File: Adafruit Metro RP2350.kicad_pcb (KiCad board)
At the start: 4 copper layers, 55 x 65.6 mm, 64 parts, among them J1 USB_C_Receptacle_USB2.0_14P, J2 Conn_02x09_Counter_Clockwise, J3 Conn_01x05_Pin, SW2 SW_RA, SW3 SW_RA, U1 APS1604M-3SQRx-SN, U2 W25Q128JVS, U4 74LVC1G19, U5 NCP1117-3.3_SOT223, U7 APS1604M-3SQRx-SN, X4 RP2350B, Y1 12MHz_10pF_50ohm

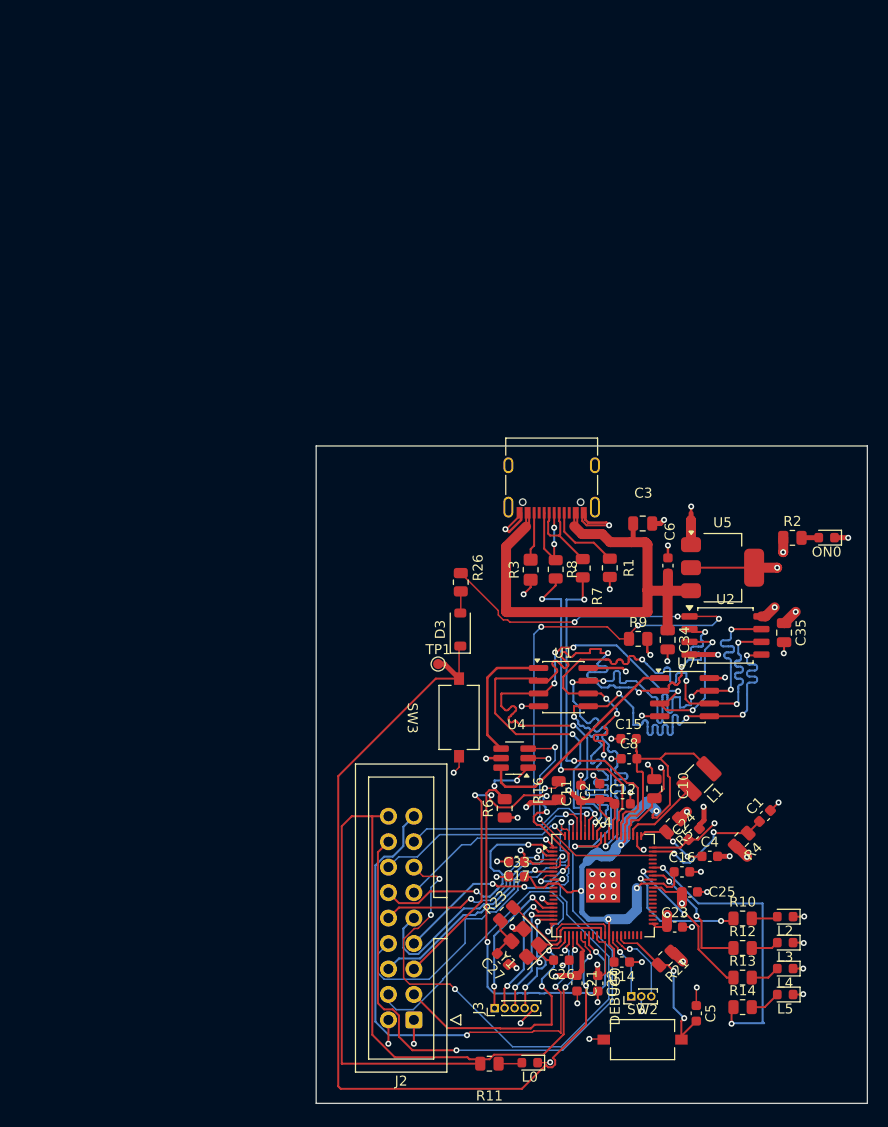
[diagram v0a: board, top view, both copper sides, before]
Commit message: Add files via upload
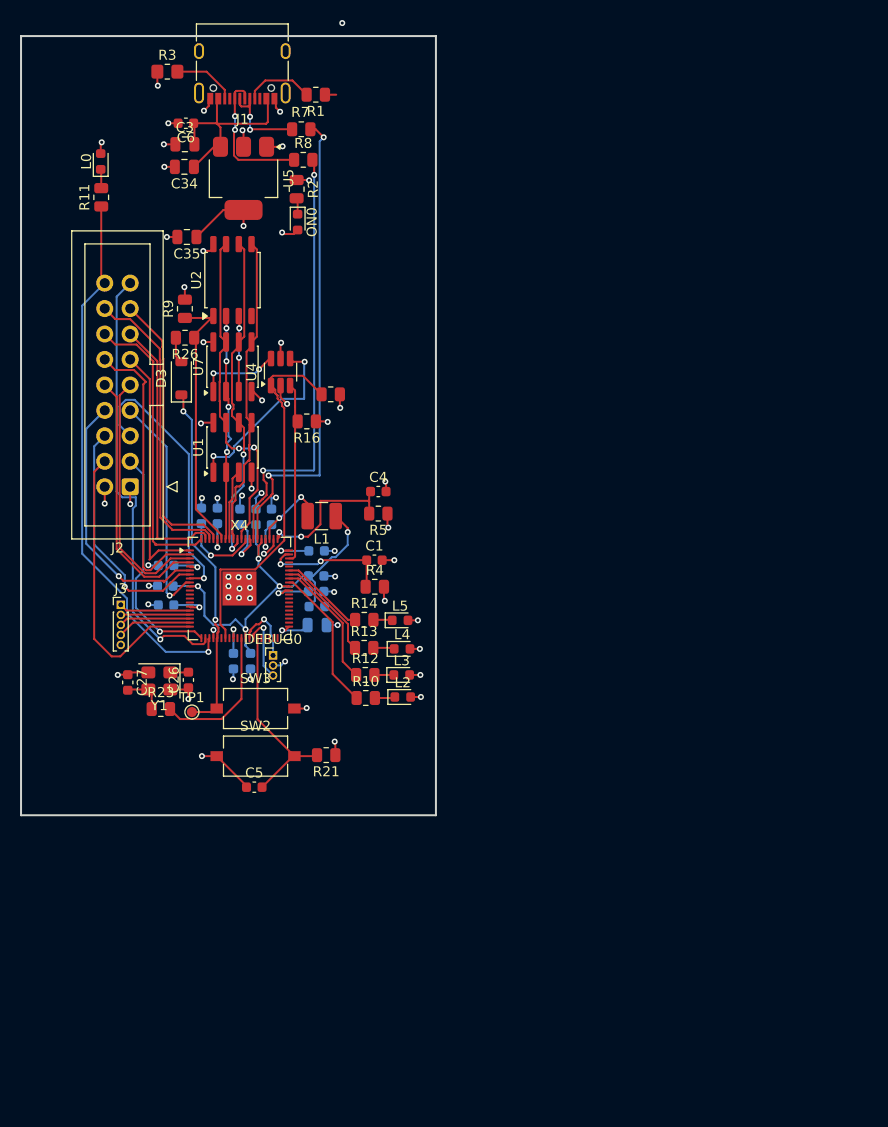
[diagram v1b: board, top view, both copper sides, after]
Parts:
- C10, C11, C12, C14, C15, C16, C17, C2, C21, C22, C23, C24, C25, C33, C8: moved to B.Cu
- moved L0 99.6 mm to (28.5, 33.6), turned to 90 degrees
- moved R11 94.7 mm to (28.6, 37.2), turned to 90 degrees
- moved C35 71.5 mm to (37.1, 41.2), turned to 180 degrees
- moved C34 67.5 mm to (36.9, 34.2), turned to 180 degrees
- moved C6 65.3 mm to (37.0, 29.8), turned to 180 degrees
- moved U5 61.6 mm to (42.8, 35.3), turned to -90 degrees
- moved R3 61.5 mm to (35.1, 24.7), turned to 0 degrees
- moved ON0 61.5 mm to (48.1, 39.7), turned to -90 degrees
- moved U2 60.6 mm to (41.6, 45.5), turned to 90 degrees
- moved R2 60.5 mm to (48.0, 36.4), turned to -90 degrees
- moved J2 60.3 mm to (31.4, 66.1)
- moved C22 60.1 mm to (40.1, 69.0), turned to 90 degrees
- moved C23 60.1 mm to (35.0, 77.9), turned to 180 degrees
- moved C3 59.3 mm to (36.9, 31.9), turned to 0 degrees
- moved C21 57.4 mm to (42.4, 69.1), turned to 90 degrees
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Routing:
- net /USBBOOT: track 91.3 -> 35.5 mm
- net /QSPI_DATA[2]: track 65.3 -> 14.6 mm, vias 8 -> 2
- net /QSPI_CS: track 76.0 -> 26.9 mm, vias 6 -> 0
- net /QSPI_DATA[1]: track 68.9 -> 22.2 mm, vias 6 -> 4
- net /PD: track 95.9 -> 54.7 mm, vias 2 -> 1
- net /D5: track 64.2 -> 27.2 mm, vias 4 -> 0
- net /D2: track 66.3 -> 30.1 mm, vias 2 -> 0
- net VBUS: track 56.2 -> 20.4 mm
- net /QSPI_DATA[3]: track 68.1 -> 33.3 mm, vias 6 -> 2
- net /QSPI_DATA[0]: track 64.9 -> 30.9 mm, vias 6 -> 0
- net /QSPI_SCK: track 66.4 -> 33.0 mm, vias 8 -> 2
- net 1.2V: track 70.8 -> 46.6 mm
- net 3.3V: track 91.4 -> 67.4 mm, vias 23 -> 25
- net GND: track 83.2 -> 60.7 mm, vias 56 -> 50
- net /A3: track 29.5 -> 8.63 mm, vias 2 -> 0
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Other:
- board size 55 x 65.6 mm -> 41.4 x 77.8 mm
- board text removed: "X4"
